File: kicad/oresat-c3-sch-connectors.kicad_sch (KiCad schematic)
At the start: 18 parts, among them J1 Conn_02x26_Odd_Even, J2 Conn_02x26_Odd_Even, J7 2-1734592-0

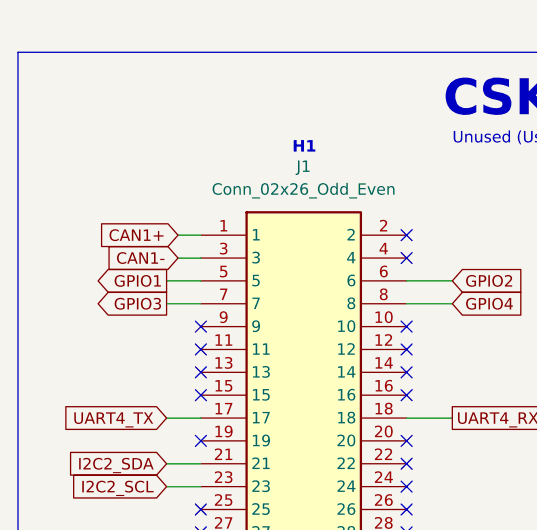
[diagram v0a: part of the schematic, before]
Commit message: Finished rerouting CAN
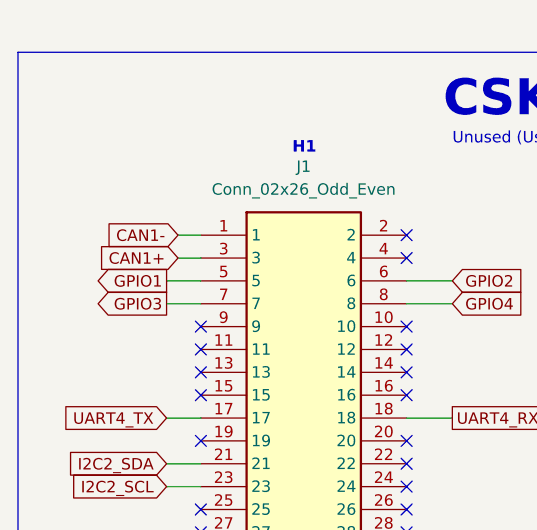
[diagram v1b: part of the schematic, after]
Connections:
- net CAN1+: now also J1.3; no longer J1.1
- net CAN1-: now also J1.1; no longer J1.3
